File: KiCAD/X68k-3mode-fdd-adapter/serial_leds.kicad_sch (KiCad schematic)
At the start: 4 parts

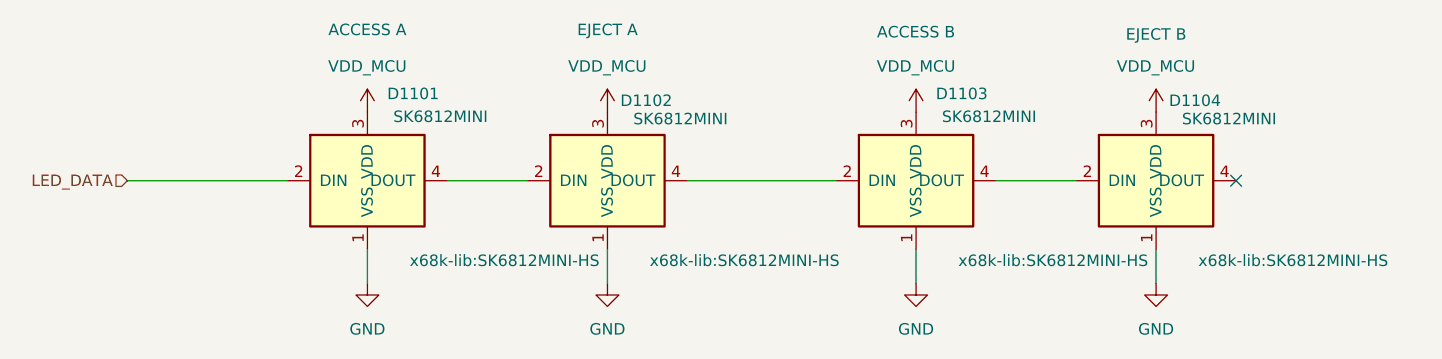
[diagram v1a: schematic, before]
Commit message: V2.1.0の基板を引き切った
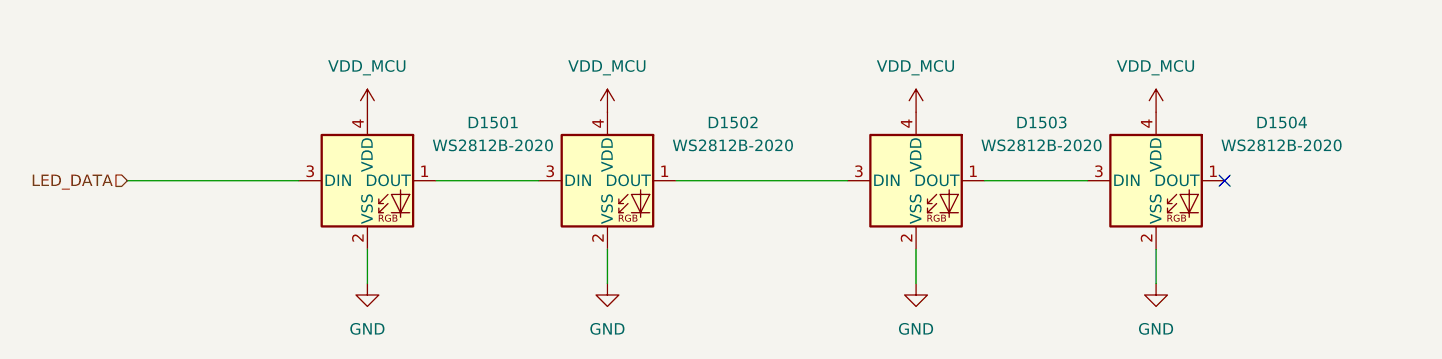
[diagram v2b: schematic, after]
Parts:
- removed D1101, D1102, D1103, D1104: SK6812MINI, x68k-lib:SK6812MINI-HS, symbol x68000-ext:SK6812MINI-HS
- added D1501, D1502, D1503, D1504: WS2812B-2020, LED_SMD:LED_WS2812B-2020_PLCC4_2.0x2.0mm, symbol LED:WS2812B-2020
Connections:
- net GND: now also D1501.2 (VSS), D1502.2 (VSS), D1503.2 (VSS), D1504.2 (VSS)
- net LED_DATA: now also D1501.3 (DIN)
- net VDD_MCU: now also D1501.4 (VDD), D1502.4 (VDD), D1503.4 (VDD), D1504.4 (VDD)
- new net: D1502.1 (DOUT), D1503.3 (DIN)
- new net: D1501.1 (DOUT), D1502.3 (DIN)
- new net: D1503.1 (DOUT), D1504.3 (DIN)
